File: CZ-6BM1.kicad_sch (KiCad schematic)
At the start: 89 parts, among them IC1 74LS245, IC10 74LS393, IC11 74LS74, IC12 74ALS00, IC13 74LS00, IC14 74LS07, IC15 74LS157, IC16 NJM2903D, IC2 S260, IC3 74LS133, IC4 74LS08, IC5 74LS38, IC6 ym3802-x, IC7 74LS32, IC8 74LS04, IC9 74LS10, J1 x68000_expansion, J2 Mini-DIN-5 (out), J3 Mini-DIN-5 (through), J4 Mini-DIN-5 (IN), J5 Conn_Coaxial (sync in), J6 Conn_Coaxial (sync out), X1 16MHz, X2 4.9152MHz

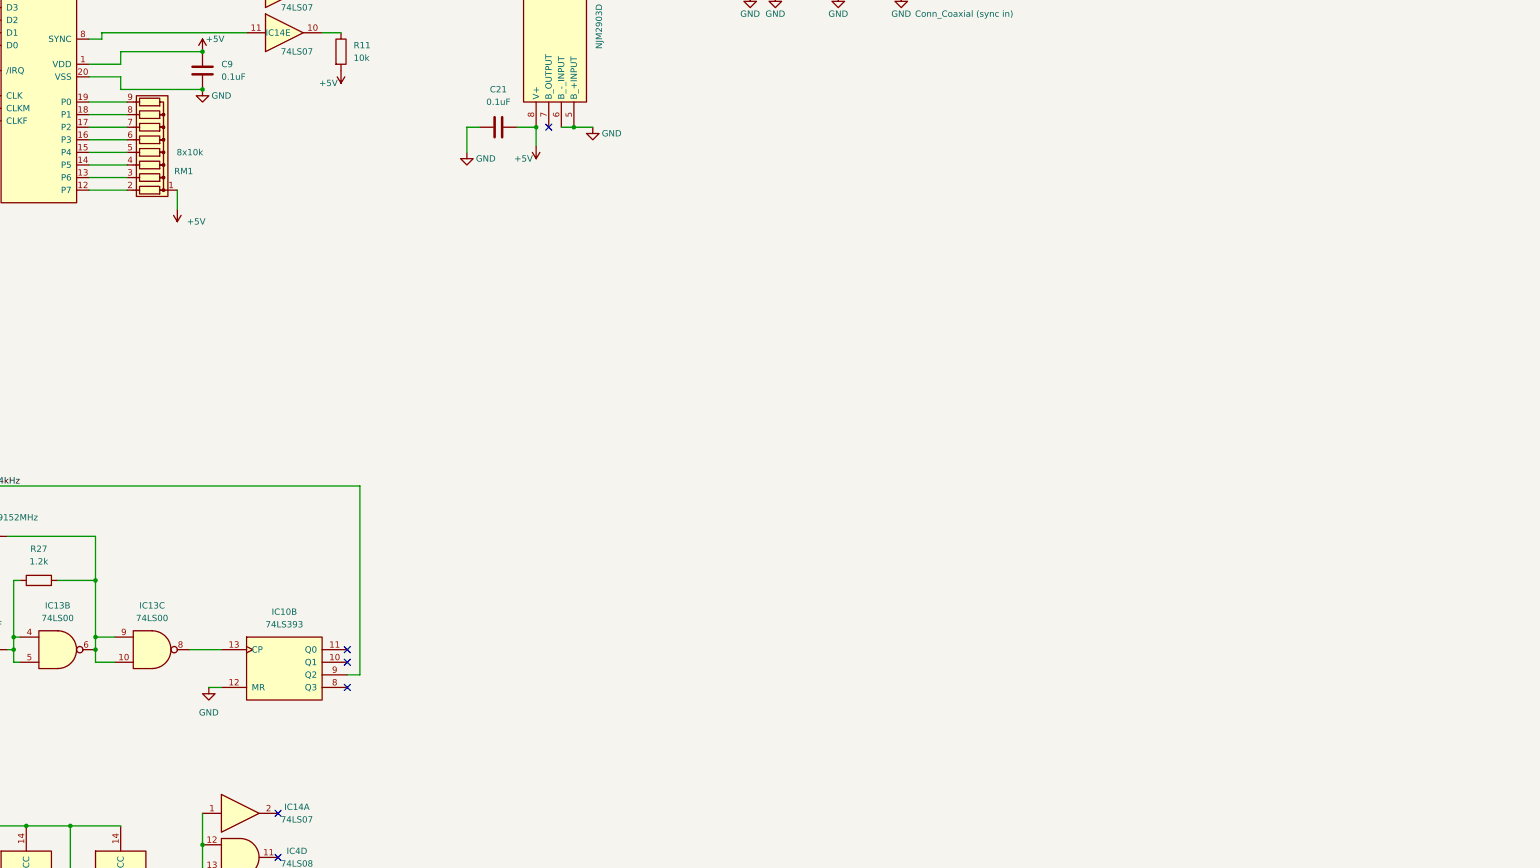
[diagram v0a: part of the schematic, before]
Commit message: mk2
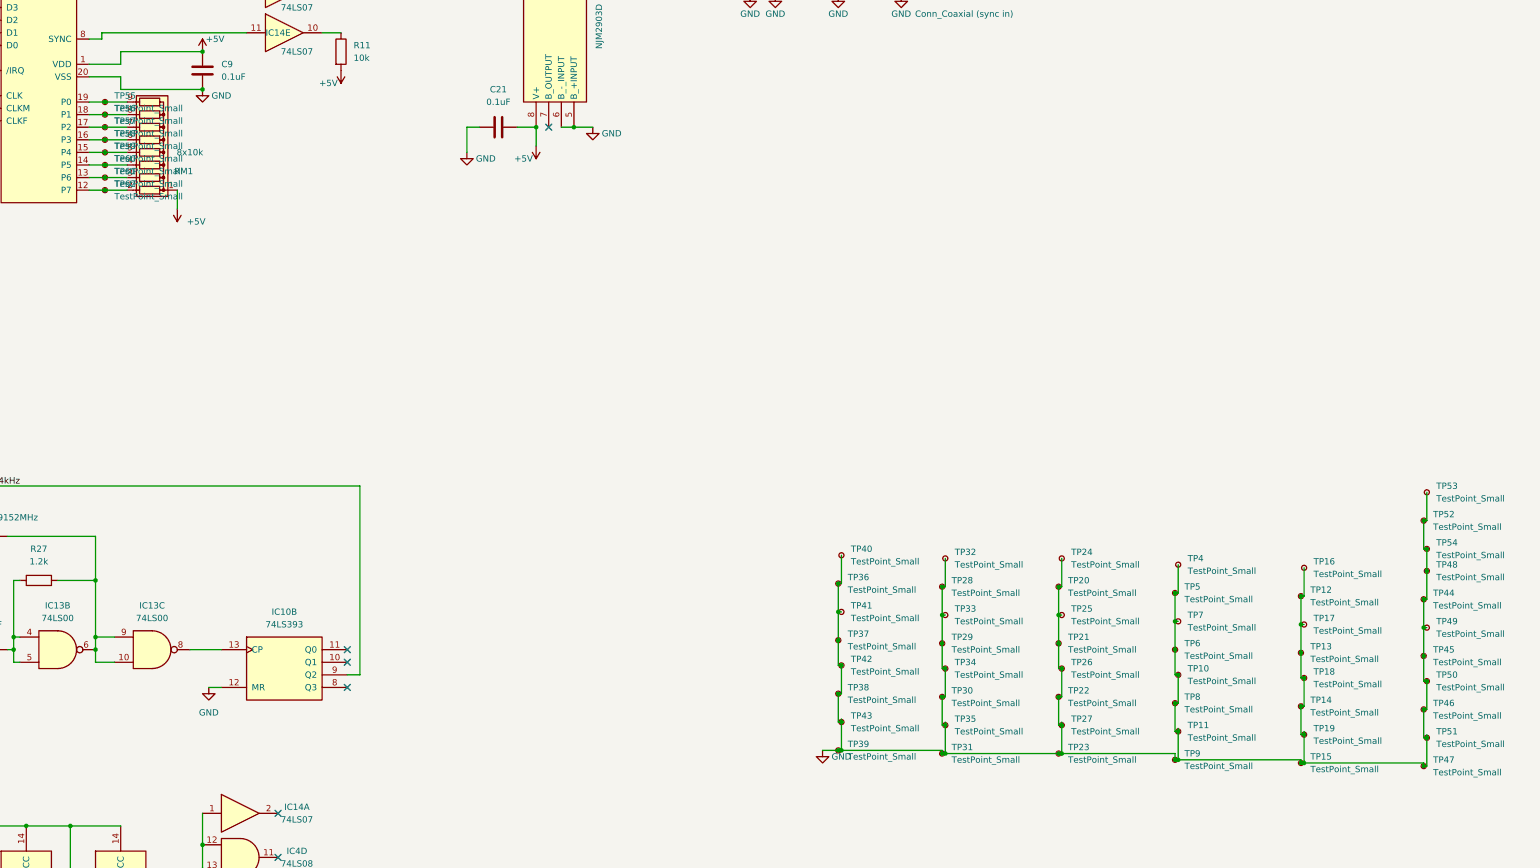
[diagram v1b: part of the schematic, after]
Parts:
- added TP10, TP11, TP12, TP13, TP14, TP15, TP16, TP17, TP18, TP19, TP20, TP21, TP22, TP23, TP24, TP25, TP26, TP27, TP28, TP29, TP30, TP31, TP32, TP33, TP34, TP35, TP36, TP37, TP38, TP39, TP4, TP40, TP41, TP42, TP43, TP44, TP45, TP46, TP47, TP48, TP49, TP5, TP50, TP51, TP52, TP53, TP54, TP55, TP56, TP57, TP58, TP59, TP6, TP60, TP61, TP62, TP7, TP8, TP9: TestPoint_Small, CustomMountingHole:TestPoint_THTPad_D1.0mm_Drill0.5mm, symbol Connector:TestPoint_Small
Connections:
- net GND: now also TP10.1, TP11.1, TP12.1, TP13.1, TP14.1, TP15.1, TP16.1, TP17.1, TP18.1, TP19.1, TP20.1, TP21.1, TP22.1, TP23.1, TP24.1, TP25.1, TP26.1, TP27.1, TP28.1, TP29.1, TP30.1, TP31.1, TP32.1, TP33.1, TP34.1, TP35.1, TP36.1, TP37.1, TP38.1, TP39.1, TP4.1, TP40.1, TP41.1, TP42.1, TP43.1, TP44.1, TP45.1, TP46.1, TP47.1, TP48.1, TP49.1, TP5.1, TP50.1, TP51.1, TP52.1, TP53.1, TP54.1, TP6.1, TP7.1, TP8.1, TP9.1
- net at IC6.12 (P7), RM1.2 (R1): now also TP62.1
- net at IC6.13 (P6), RM1.3 (R2): now also TP61.1
- net at IC6.14 (P5), RM1.4 (R3): now also TP60.1
- net at IC6.15 (P4), RM1.5 (R4): now also TP59.1
- net at IC6.16 (P3), RM1.6 (R5): now also TP58.1
- net at IC6.17 (P2), RM1.7 (R6): now also TP57.1
- net at IC6.18 (P1), RM1.8 (R7): now also TP56.1
- net at IC6.19 (P0), RM1.9 (R8): now also TP55.1
